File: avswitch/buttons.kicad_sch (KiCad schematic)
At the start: 21 parts, among them J701 CTRL, J703 Conn_01x02, J704 Conn_01x04

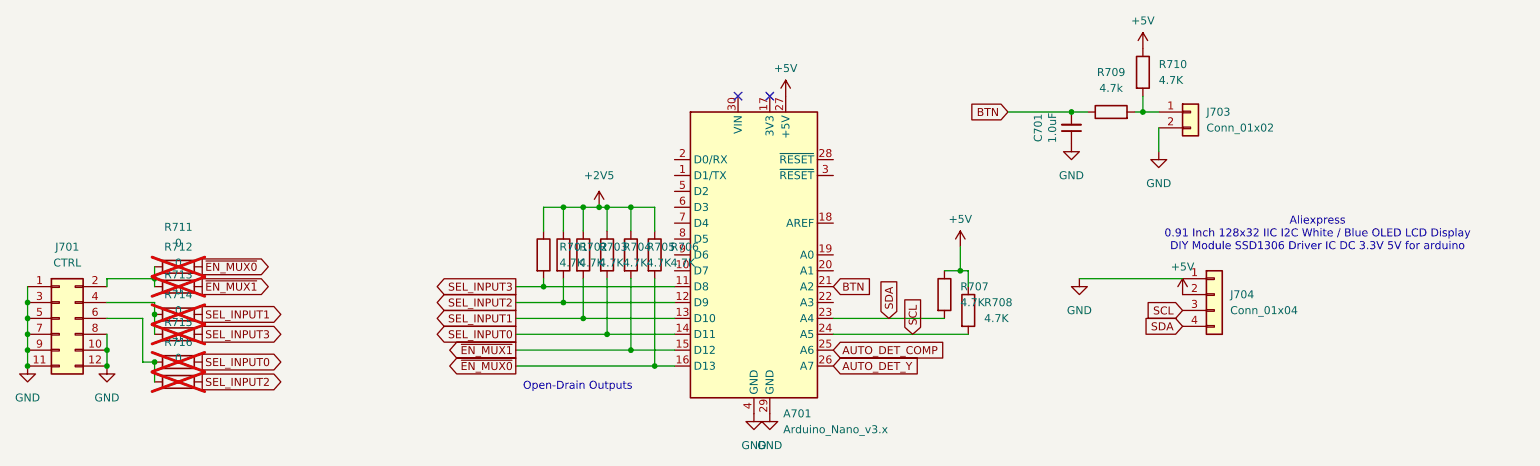
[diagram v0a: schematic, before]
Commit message: PCB Layout nearing completion
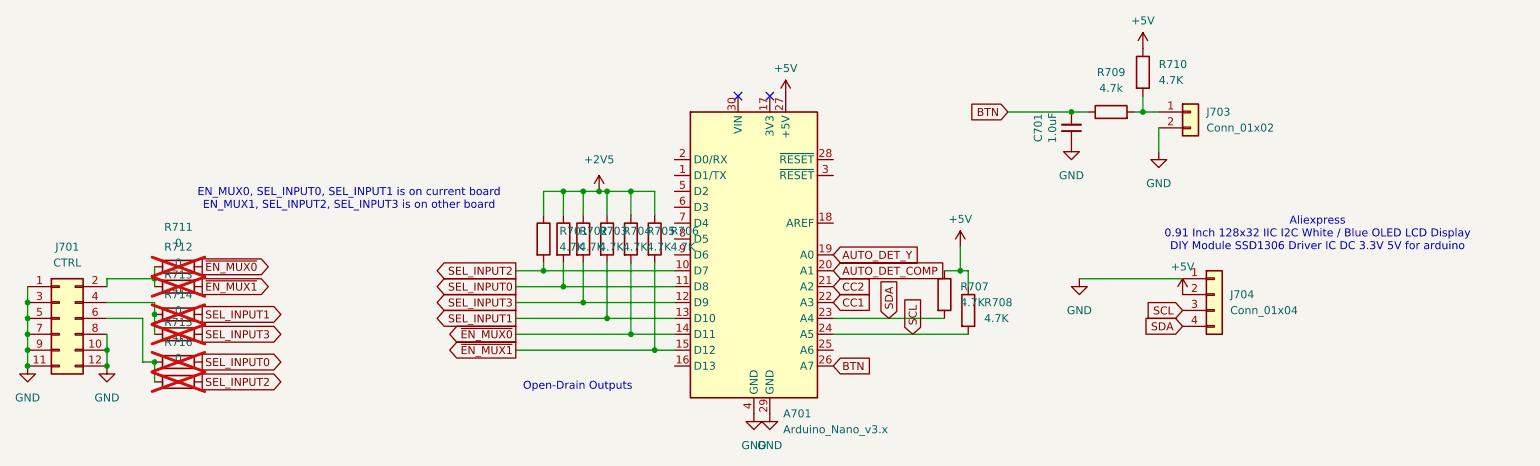
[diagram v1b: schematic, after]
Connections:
- net AUTO_DET_COMP: now also A701.20 (A1); no longer A701.25 (A6)
- net AUTO_DET_Y: now also A701.19 (A0); no longer A701.26 (A7)
- net BTN: now also A701.26 (A7); no longer A701.21 (A2)
- net SEL_INPUT0: now also A701.11 (D8), R702.2; no longer A701.14 (D11), R704.2
- net SEL_INPUT1: now also R704.2; no longer R703.2
- net SEL_INPUT2: now also A701.10 (D7), R701.2; no longer A701.12 (D9), R702.2
- net SEL_INPUT3: now also A701.12 (D9), R703.2; no longer A701.11 (D8), R701.2
- net ~{EN_MUX0}: now also A701.14 (D11), R705.2; no longer A701.16 (D13), R706.2
- net ~{EN_MUX1}: now also R706.2; no longer R705.2
- net CC1: now reaches A701.22 (A3)
- new net CC2: A701.21 (A2)
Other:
- note added: "EN_MUX0, SEL_INPUT0, SEL_INPUT1 is on current board EN_MUX1, SEL_INPUT2, SEL_INPUT3 is on other board"
- moved on the sheet: R701, R702, R703, R704, R705, R706
